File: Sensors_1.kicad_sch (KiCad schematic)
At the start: 21 parts, among them J7 Conn_01x04_Pin, J8 Conn_01x04_Pin, U3 Ai-Thinker-Ra-01

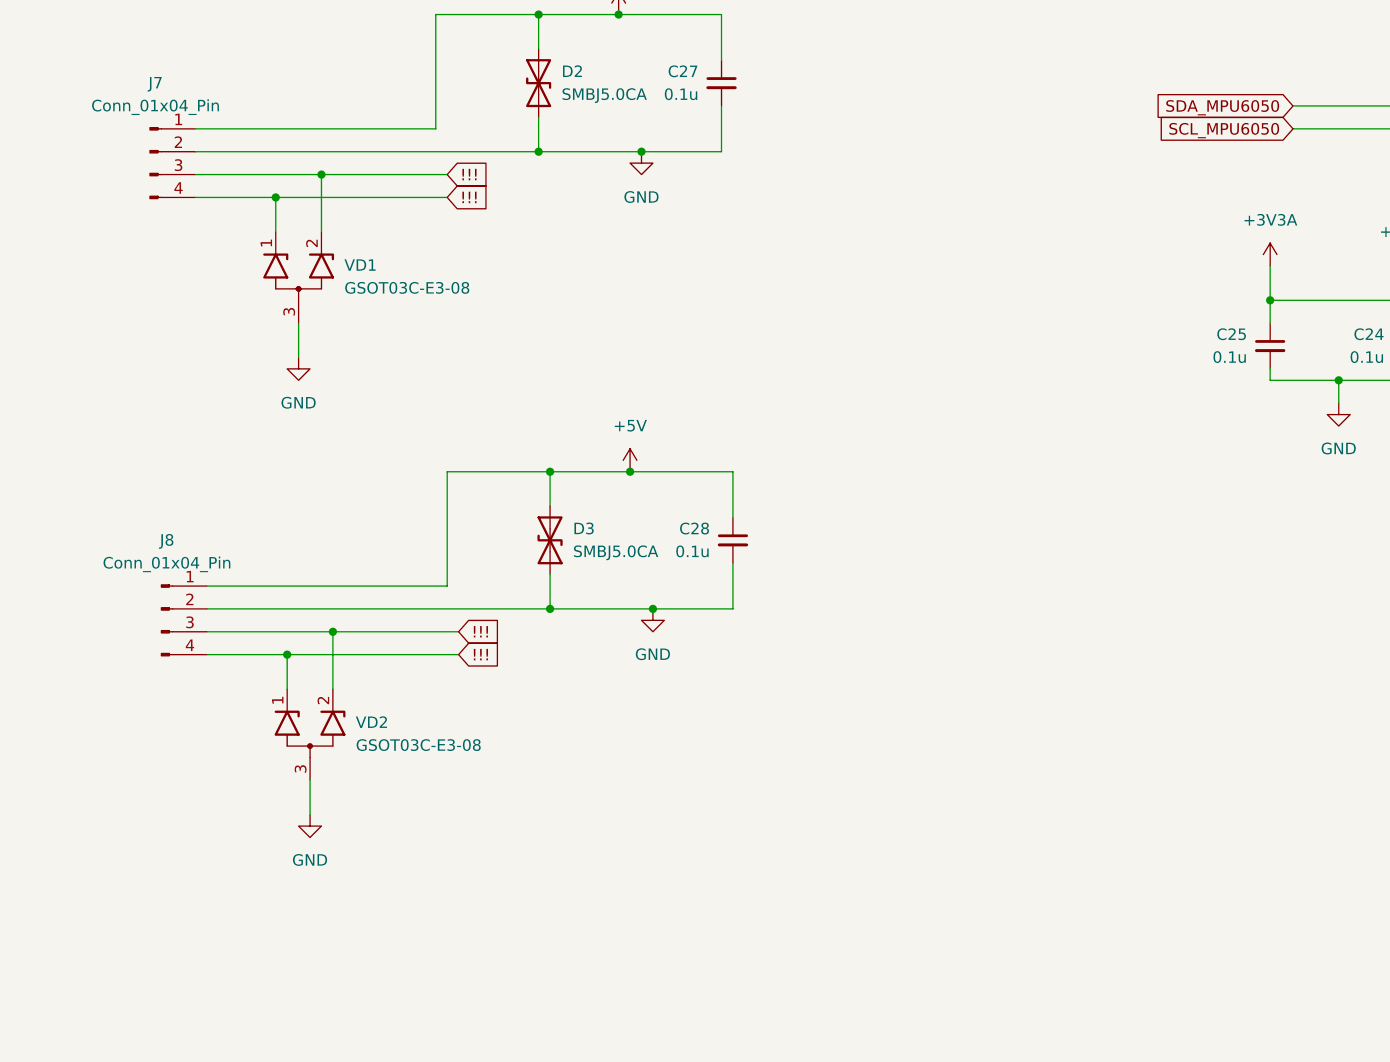
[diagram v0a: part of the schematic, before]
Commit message: feat: firs complete version schemattic
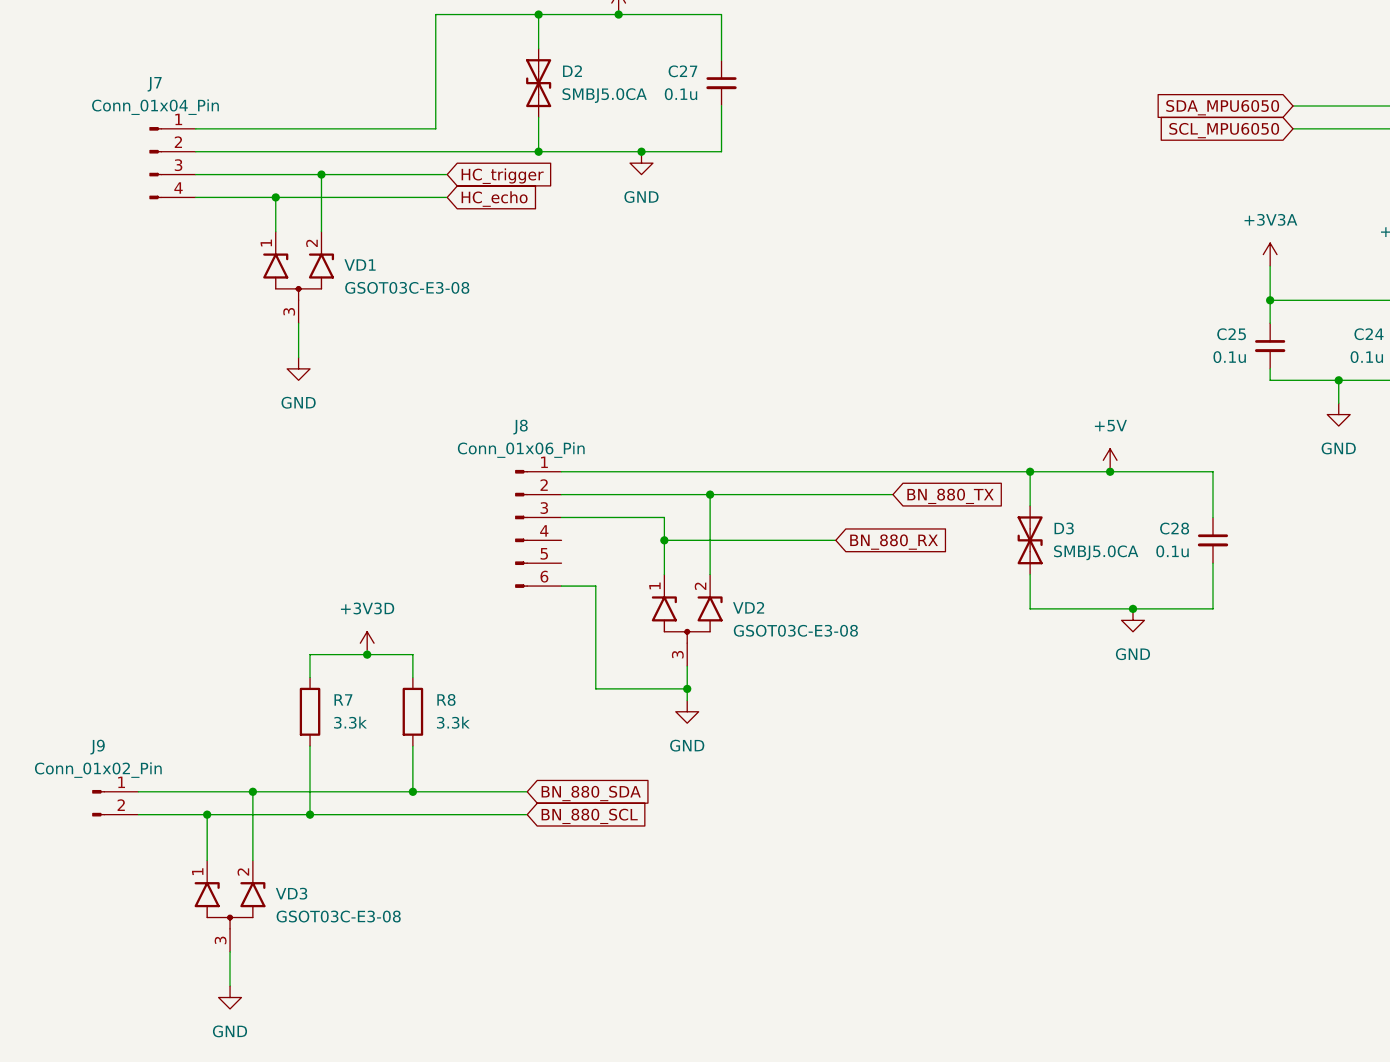
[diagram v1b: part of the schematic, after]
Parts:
- removed J8: Conn_01x04_Pin, Connector_PinHeader_2.54mm:PinHeader_1x04_P2.54mm_Horizontal, symbol Connector:Conn_01x04_Pin
- added J8: Conn_01x06_Pin, Connector_Hirose:Hirose_DF13-06P-1.25DSA_1x06_P1.25mm_Vertical, symbol Connector:Conn_01x06_Pin
- added J9: Conn_01x02_Pin, Connector_Hirose:Hirose_DF13-02P-1.25DSA_1x02_P1.25mm_Vertical, symbol Connector:Conn_01x02_Pin
- added R7, R8: 3.3k, Resistor_SMD:R_0805_2012Metric_Pad1.20x1.40mm_HandSolder, symbol Device:R
- added VD3: GSOT03C-E3-08, Package_TO_SOT_SMD:SOT-23_Handsoldering, symbol TWS:GSOT03C-E3-08
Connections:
- net +3V3D: now also R7.1, R8.1
- net +5V: now also J8.1 (Pin_1)
- net GND: now also J8.6 (Pin_6), VD3.3 (A)
- removed net !!!: J7.3 (Pin_3), J7.4 (Pin_4), VD1.1 (K1), VD1.2 (K2), VD2.1 (K1), VD2.2 (K2)
- new net BN_880_RX: J8.3 (Pin_3), VD2.1 (K1)
- new net BN_880_SCL: J9.2 (Pin_2), R7.2, VD3.1 (K1)
- new net BN_880_SDA: J9.1 (Pin_1), R8.2, VD3.2 (K2)
- new net BN_880_TX: J8.2 (Pin_2), VD2.2 (K2)
- new net HC_echo: J7.4 (Pin_4), VD1.1 (K1)
- new net HC_trigger: J7.3 (Pin_3), VD1.2 (K2)
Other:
- moved on the sheet: C28, D3, VD2
